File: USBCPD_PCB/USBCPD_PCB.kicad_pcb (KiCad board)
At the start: 2 copper layers, 64 parts, among them IC1 TMCS1108A3BQDRQ1, IC2 UCC27282QDRQ1, IC3 UCC27282QDRQ1, IC4 BAJ2CC0FP-E2, J1 TB002-500-02BE, J2 TB002-500-02BE, Q1 SIR584DP-T1-RE3, Q2 SIR584DP-T1-RE3, Q3 SIR584DP-T1-RE3, Q4 SIR584DP-T1-RE3, U1 NUCLEO-G474RE

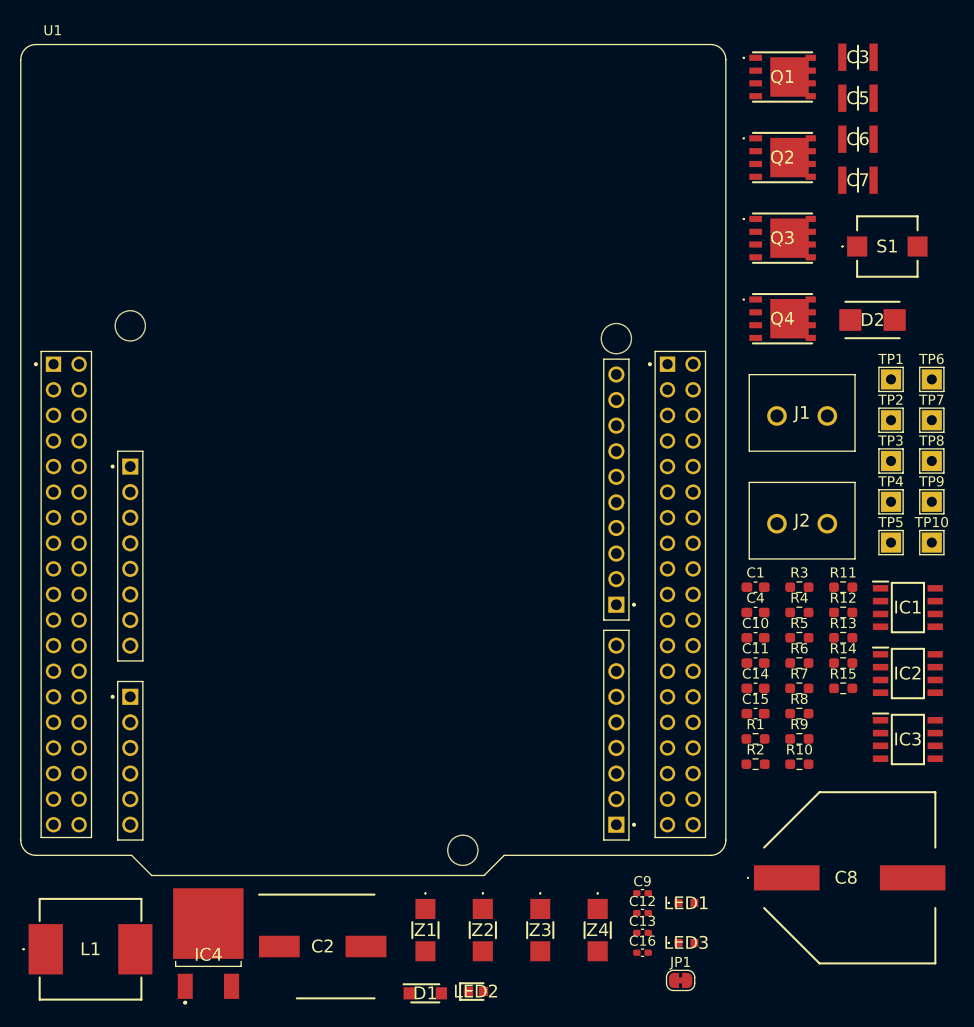
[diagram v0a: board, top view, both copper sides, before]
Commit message: PCB layout, components sorted
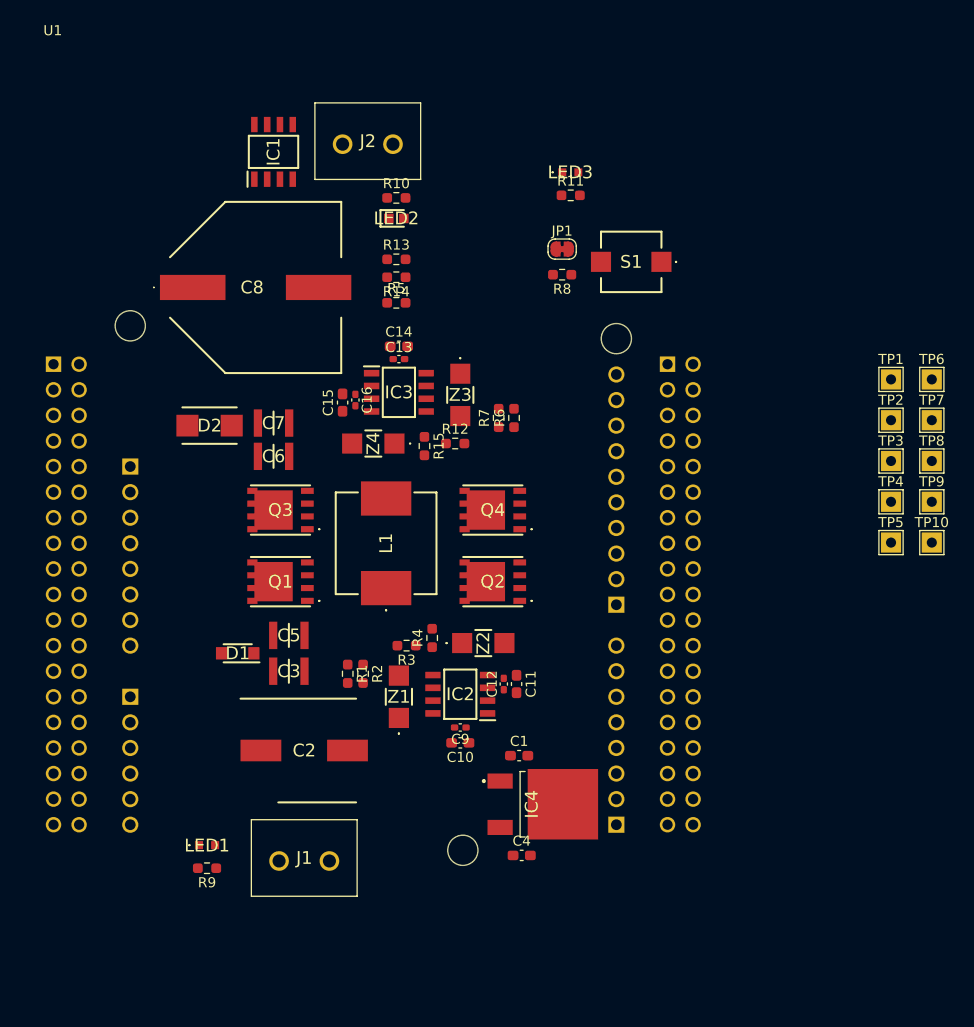
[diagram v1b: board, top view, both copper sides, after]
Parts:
- moved C8 83.2 mm to (129.3, 71.1)
- moved C3 83.1 mm to (132.6, 109.2), turned to 180 degrees
- moved C5 77.7 mm to (132.6, 105.7), turned to 180 degrees
- moved IC1 77.5 mm to (131.1, 57.7), turned to 90 degrees
- moved LED3 77.4 mm to (160.5, 59.7)
- moved LED2 77.2 mm to (143.3, 64.3)
- moved JP1 73.6 mm to (159.7, 67.3)
- moved Q1 70.7 mm to (131.8, 100.3), turned to 180 degrees
- moved R10 69.0 mm to (143.3, 62.2)
- moved D2 66.6 mm to (124.7, 84.8)
- moved J1 66.3 mm to (131.6, 128.1)
- moved C6 66.0 mm to (131.1, 87.9), turned to 180 degrees
- moved C7 62.8 mm to (131.1, 84.6), turned to 180 degrees
- moved C13 61.9 mm to (143.5, 78.2)
- moved C16 61.8 mm to (139.2, 82.3), turned to -90 degrees
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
